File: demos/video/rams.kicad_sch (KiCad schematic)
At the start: 8 parts, among them U12 SIM4X32, U13 SIM4X32, U14 SIM4X32, U15 SIM4X32, U16 SIM4X32, U17 SIM4X32, U18 SIM4X32, U19 SIM4X32

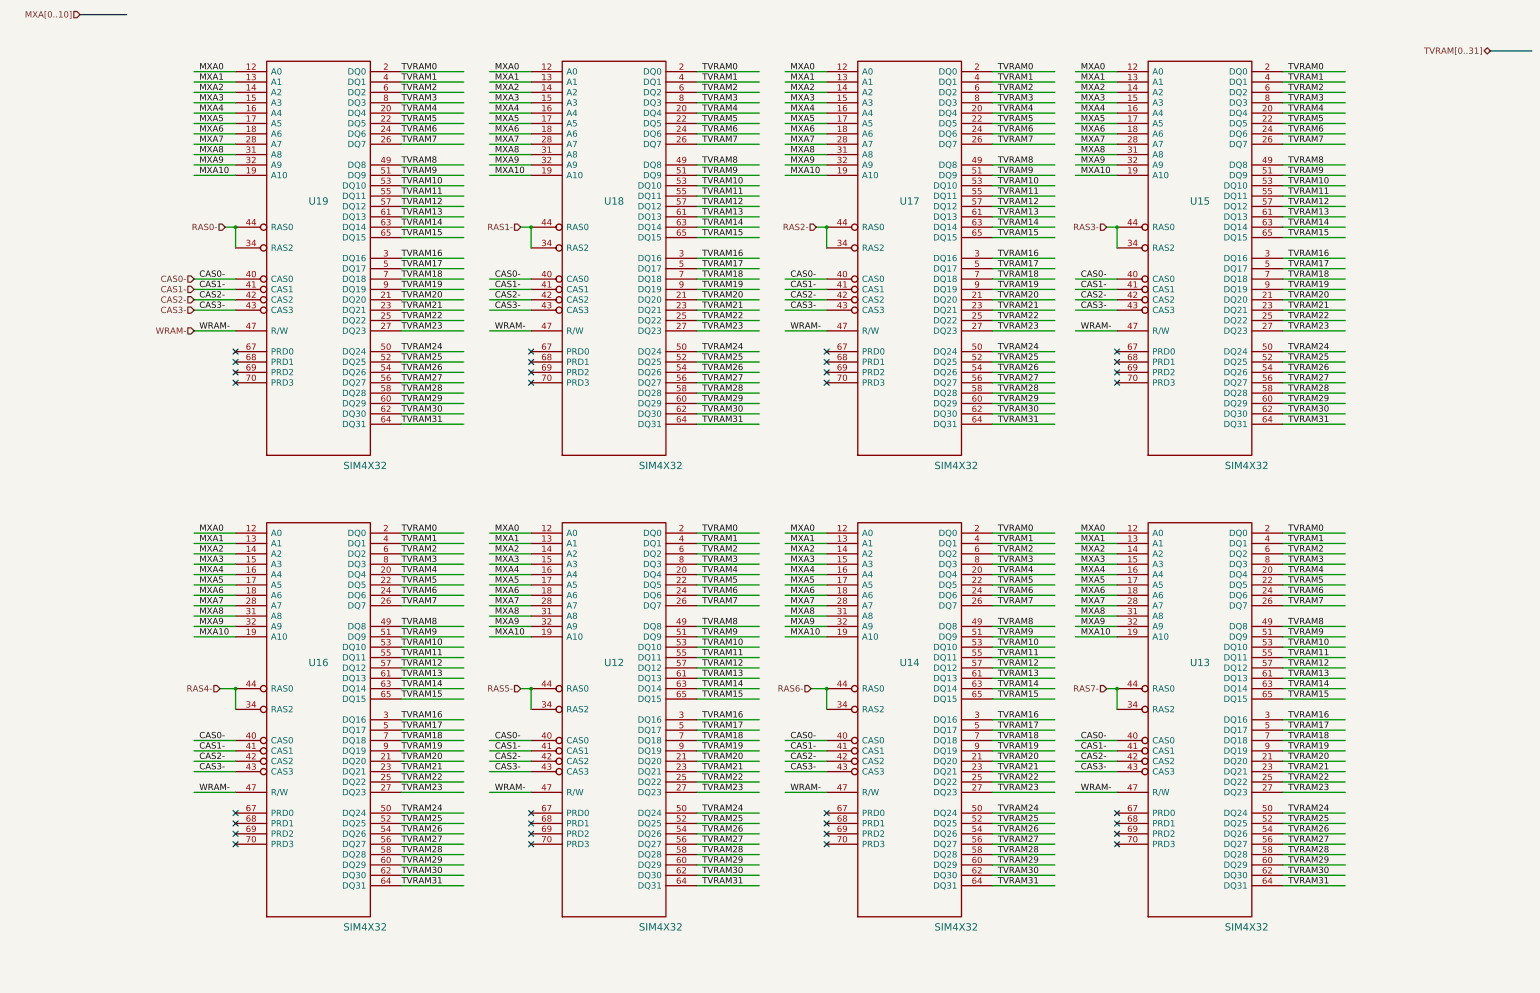
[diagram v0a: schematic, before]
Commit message: Demo update
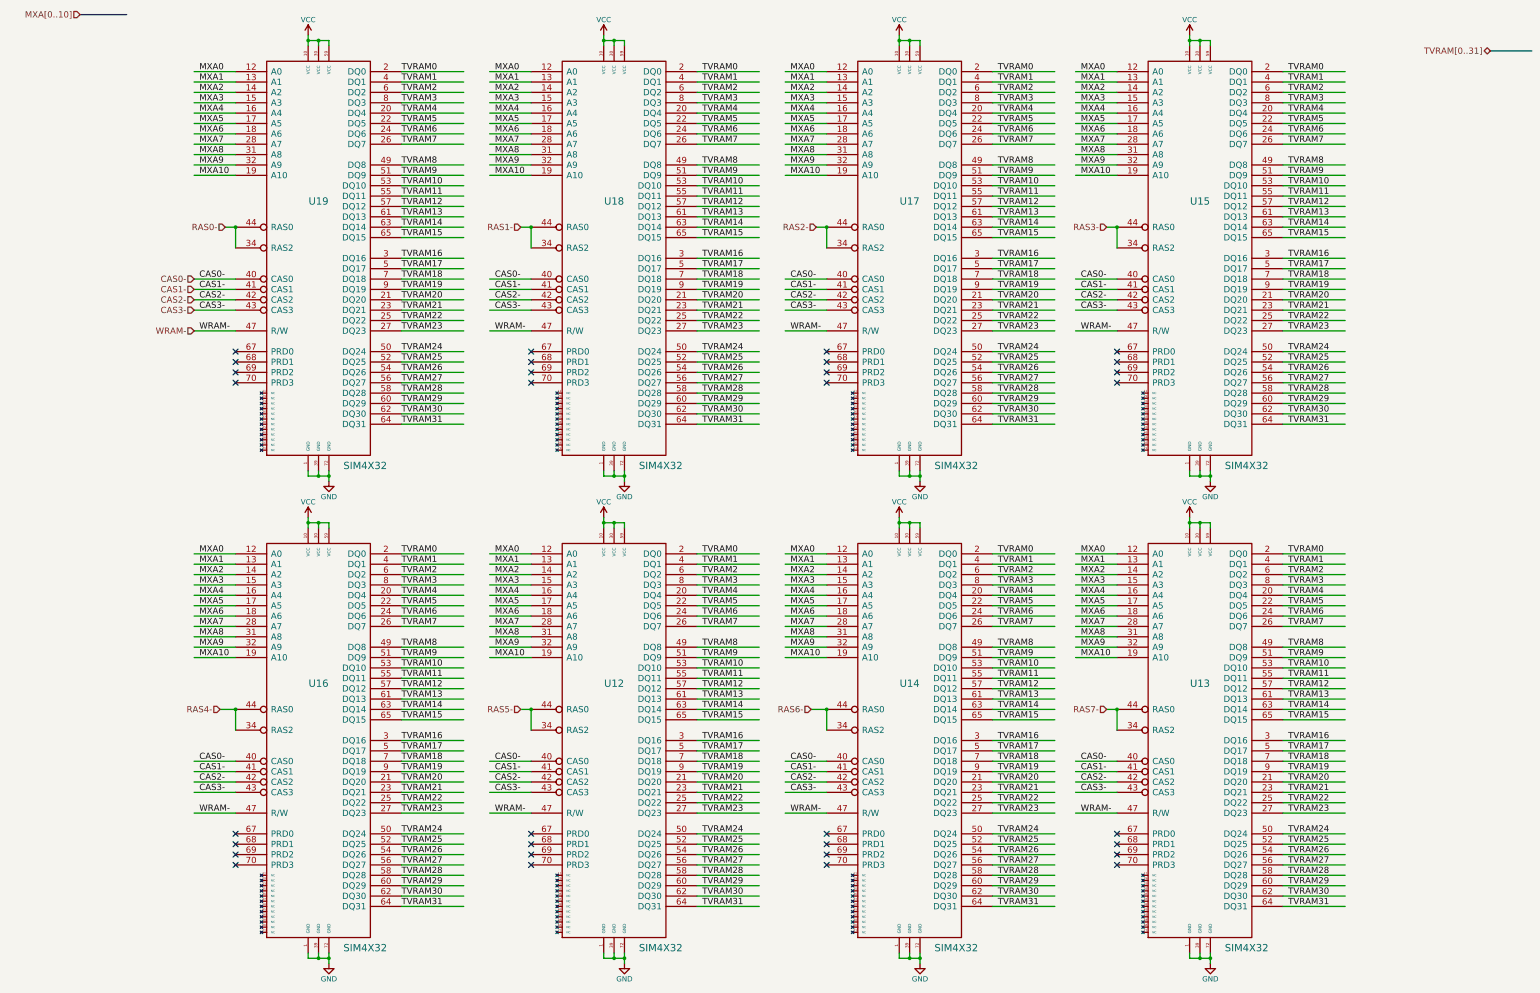
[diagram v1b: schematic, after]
